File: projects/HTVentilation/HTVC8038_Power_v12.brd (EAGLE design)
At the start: 80.6 x 58.1 mm, 71 parts

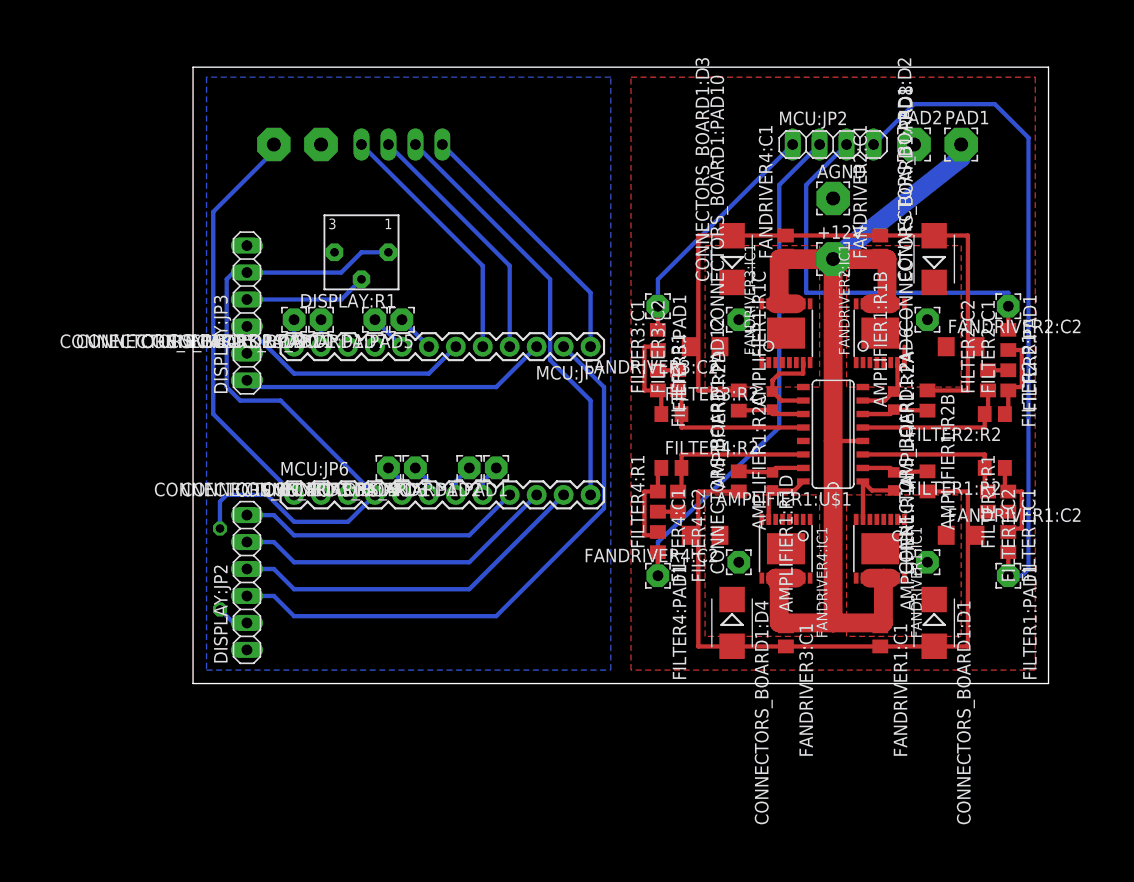
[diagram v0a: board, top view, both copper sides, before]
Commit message: cleanup
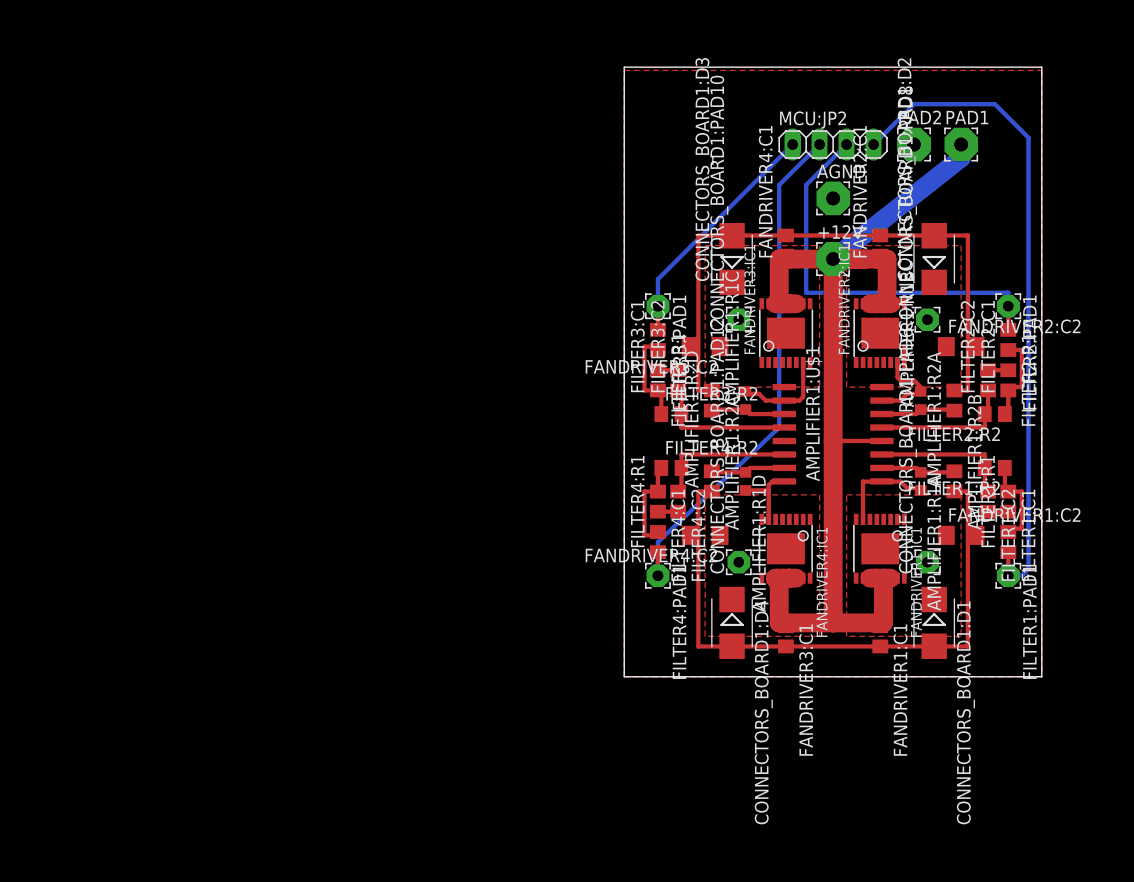
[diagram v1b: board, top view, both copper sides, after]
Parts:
- removed +12V1, AGND9: (no value), wirepad:3,17/1,3
- removed CONNECTORS_BOARD1:PAD1, CONNECTORS_BOARD1:PAD11, CONNECTORS_BOARD1:PAD2, CONNECTORS_BOARD1:PAD3, CONNECTORS_BOARD1:PAD4, CONNECTORS_BOARD1:PAD5, CONNECTORS_BOARD1:PAD7, CONNECTORS_BOARD1:PAD9: (no value), wirepad:2,15/1,0
- removed DISPLAY:JP2, DISPLAY:JP3: (no value), pinhead:1X06
- removed DISPLAY:R1: 10k, nervus:3362P
- removed DISPLAY:R2: 470R, rcl:0204/7
- removed MCU:JP1: (no value), pinhead:1X04
- removed MCU:JP6, MCU:JP7: (no value), SparkFun:1X12
- AMPLIFIER1:U$1: device nervus:SO16 -> nervus:SO16W
- moved AMPLIFIER1:R1C 2.54 mm to (52.1, 26.7)
- moved AMPLIFIER1:R1D 2.54 mm to (52.1, 19.1)
- moved AMPLIFIER1:R2C 2.54 mm to (48.9, 26.7)
- moved AMPLIFIER1:R2D 2.54 mm to (48.9, 19.1)
- moved AMPLIFIER1:R1A 2.54 mm to (68.6, 19.1)
- moved AMPLIFIER1:R1B 2.54 mm to (68.6, 26.7)
- moved AMPLIFIER1:R2A 2.54 mm to (71.8, 19.1)
- moved AMPLIFIER1:R2B 2.54 mm to (71.8, 26.7)
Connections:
- removed net +5V: DISPLAY:JP3.5, DISPLAY:R1.1, DISPLAY:R2.1, MCU:JP6.4
- removed net A0: CONNECTORS_BOARD1:PAD1.1, MCU:JP6.8
- removed net A1: CONNECTORS_BOARD1:PAD2.1, MCU:JP6.7
- removed net A2: CONNECTORS_BOARD1:PAD3.1, MCU:JP6.6
- removed net A3: CONNECTORS_BOARD1:PAD4.1, MCU:JP6.5
- removed net DISPLAY:N$1: DISPLAY:JP3.4, DISPLAY:R1.2
- removed net DISPLAY:N$2: DISPLAY:JP2.2, DISPLAY:R2.2
- removed net MCU:RESET: MCU:JP6.3
- removed net N$1: DISPLAY:JP3.3, MCU:JP7.6
- removed net N$2: DISPLAY:JP3.1, MCU:JP7.3
- removed net N$3: DISPLAY:JP2.6, MCU:JP6.9
- removed net N$4: DISPLAY:JP2.5, MCU:JP6.10
- removed net N$5: DISPLAY:JP2.4, MCU:JP6.11
- removed net N$6: DISPLAY:JP2.3, MCU:JP7.2
- removed net TACH0: CONNECTORS_BOARD1:PAD5.1, MCU:JP7.7
- removed net TACH1: CONNECTORS_BOARD1:PAD7.1, MCU:JP7.8
- removed net TACH2: CONNECTORS_BOARD1:PAD9.1, MCU:JP7.12
- removed net TACH3: CONNECTORS_BOARD1:PAD11.1, MCU:JP7.11
- net AGND: no longer AGND9.1, DISPLAY:JP2.1, DISPLAY:JP3.2, DISPLAY:JP3.6, DISPLAY:R1.3, MCU:JP6.2, MCU:JP7.10, MCU:JP7.9
- net N$21: no longer MCU:JP1.4, MCU:JP7.5
- net N$22: no longer MCU:JP1.3, MCU:JP7.4
- net N$23: no longer MCU:JP1.1, MCU:JP7.1
- net N$37: no longer MCU:JP1.2, MCU:JP6.12
- net VCC: no longer +12V1.1, MCU:JP6.1
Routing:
- net +5V: track 64.1 -> 0.00 mm
- net N$6: track 55.5 -> 0.00 mm
- net N$37: track 89.2 -> 49.4 mm
- net N$5: track 34.3 -> 0.00 mm
- net N$4: track 30.7 -> 0.00 mm
- net VCC: track 145.9 -> 115.3 mm
- net N$2: track 29.1 -> 0.00 mm
- net N$3: track 27.1 -> 0.00 mm
- net N$23: track 47.6 -> 22.7 mm
- net N$21: track 86.3 -> 62.5 mm
- net N$22: track 61.9 -> 38.1 mm
- net N$1: track 22.6 -> 0.00 mm
- net DISPLAY:N$1: track 11.6 -> 0.00 mm
- net AGND: track 132.8 -> 122.7 mm
- net TACH0: track 3.59 -> 0.00 mm
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- removed copper zone on layer 16, net AGND
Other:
- board size 80.6 x 58.1 mm -> 39.3 x 57.5 mm
